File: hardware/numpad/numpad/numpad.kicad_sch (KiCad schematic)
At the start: 26 parts, among them IC1 LD1117-3.3V-SOT223, Y1 8MHz

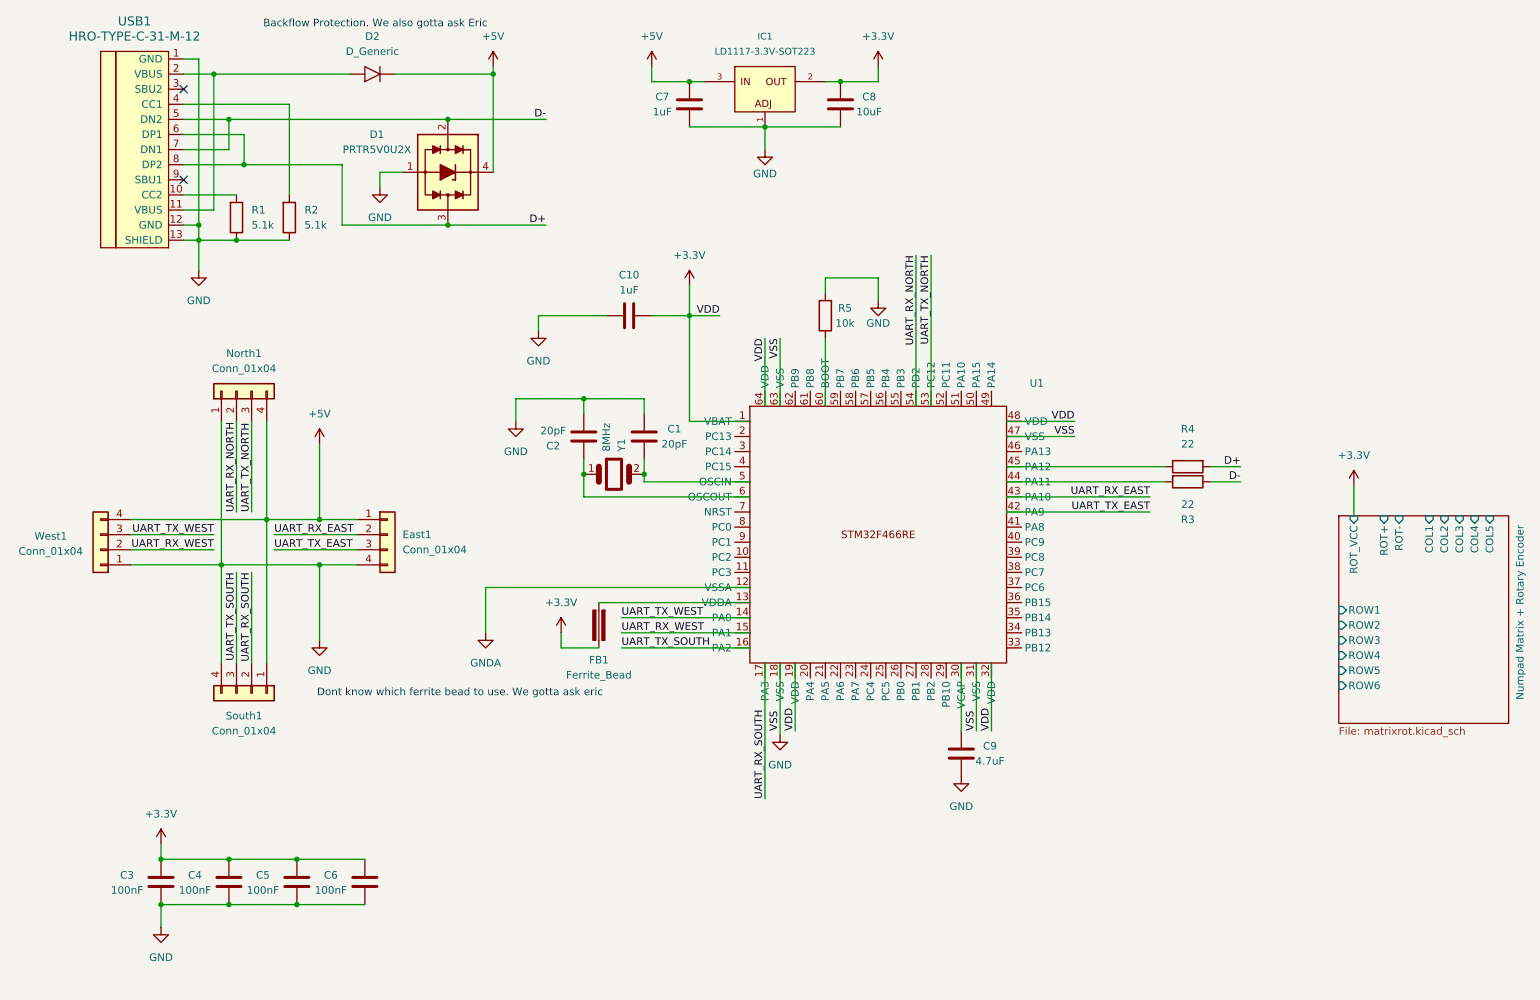
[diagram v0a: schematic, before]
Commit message: stuff
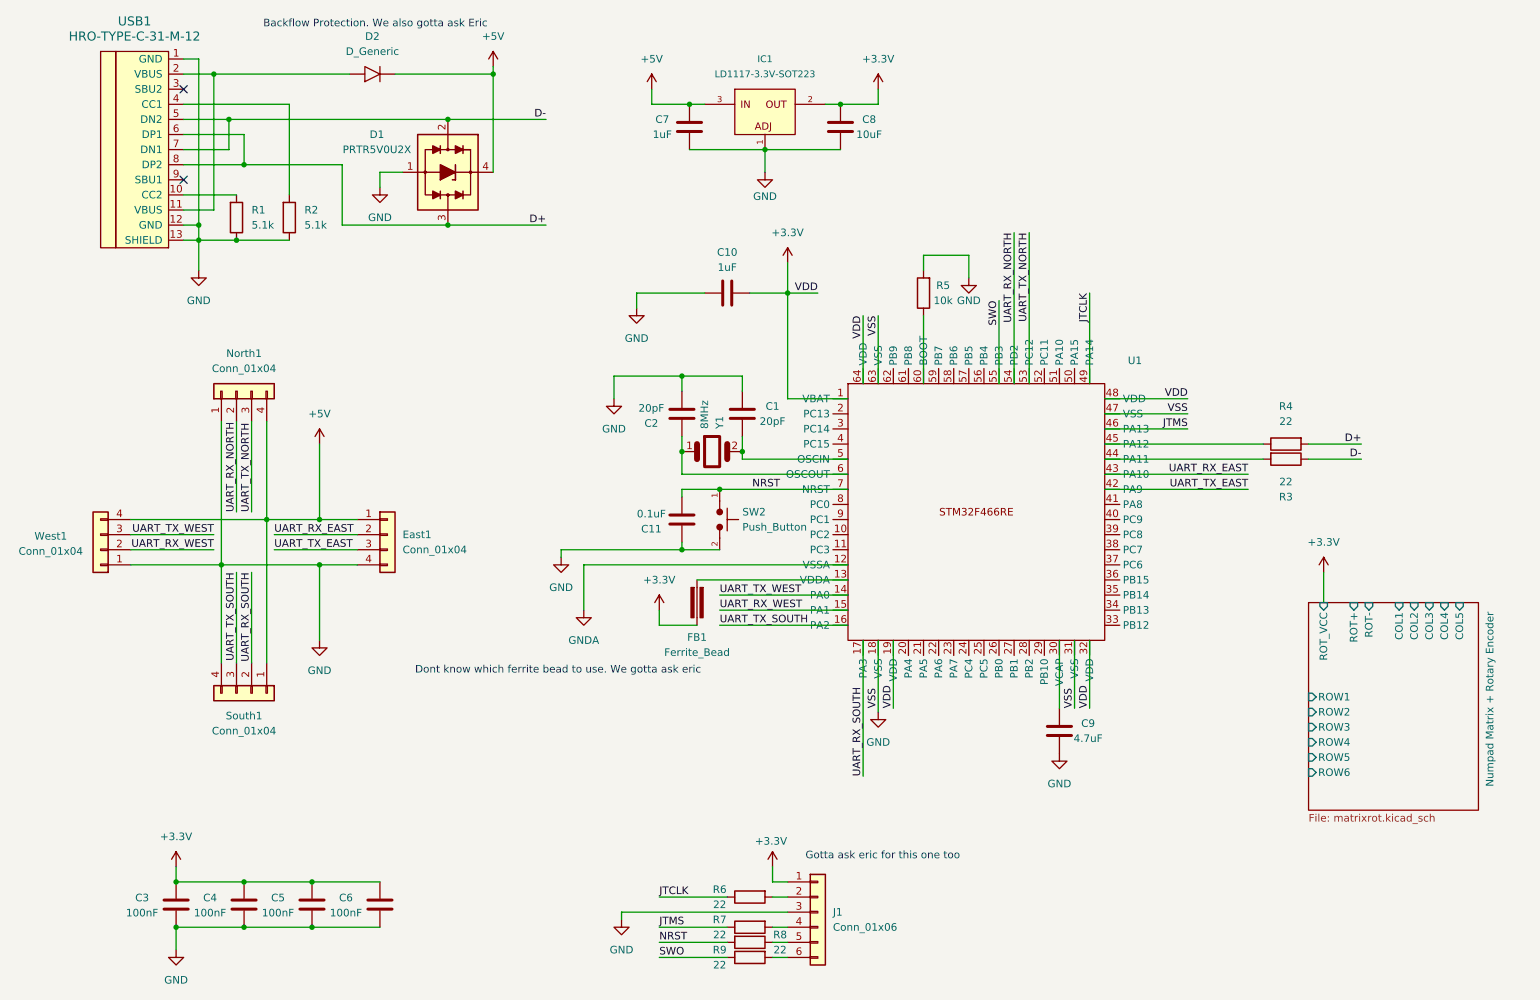
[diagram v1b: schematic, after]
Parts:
- added C11: 0.1uF, PCM_Capacitor_SMD_AKL:C_0805_2012Metric, symbol PCM_Capacitor_AKL:C_0805
- added J1: Conn_01x06, 4ms_Connector:Pins_1x06_2.54mm_TH_SWD, symbol PCM_4ms_Connector:Conn_01x06
- added R6, R7, R8, R9: 22, PCM_Resistor_SMD_AKL:R_0805_2012Metric, symbol PCM_Resistor_AKL:R_0805
- added SW2: Push_Button, Button_Switch_THT:SW_PUSH_6mm, symbol PCM_SL_Devices:Push_Button
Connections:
- net +3.3V: now also J1.1 (Pin_1)
- net GND: now also C11.1, J1.3 (Pin_3), SW2.2
- net JTMS: now reaches U1.46 (PA13)
- net JTMS: now also R7.2
- net JTCLK: now reaches U1.49 (PA14)
- net JTCLK: now also R6.2
- net SWO: now reaches U1.55 (PB3)
- net SWO: now also R9.2
- net NRST: now reaches U1.7 (NRST)
- net NRST: now also C11.2, R8.1, SW2.1
- new net: J1.4 (Pin_4), R7.1
- new net: J1.5 (Pin_5), R8.2
- new net: J1.2 (Pin_2), R6.1
- new net: J1.6 (Pin_6), R9.1
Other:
- note added: "Gotta ask eric for this one too"
- moved on the sheet: C1, C10, C2, C3, C4, C5, C6, C7, C8, C9, FB1, IC1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
